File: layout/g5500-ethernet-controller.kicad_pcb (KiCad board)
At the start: 2 copper layers, 58 parts, among them IC1 MAX-M8Q, J1 CONN_01x03, J2 CONN_01x03, J3 MICROUSB, J4 CONN_01x02, J5 CONN_01x03, J6 CONN_01x03, K1 G5LE-1, K2 G5LE-1, K3 G5LE-1, K4 G5LE-1, P1 COAX, Q1 BC817W, Q2 BC817W, Q3 BC817W, Q4 BC817W, U1 NUCLEO144-F429ZI, U2 LD3985G33R_TSOT23

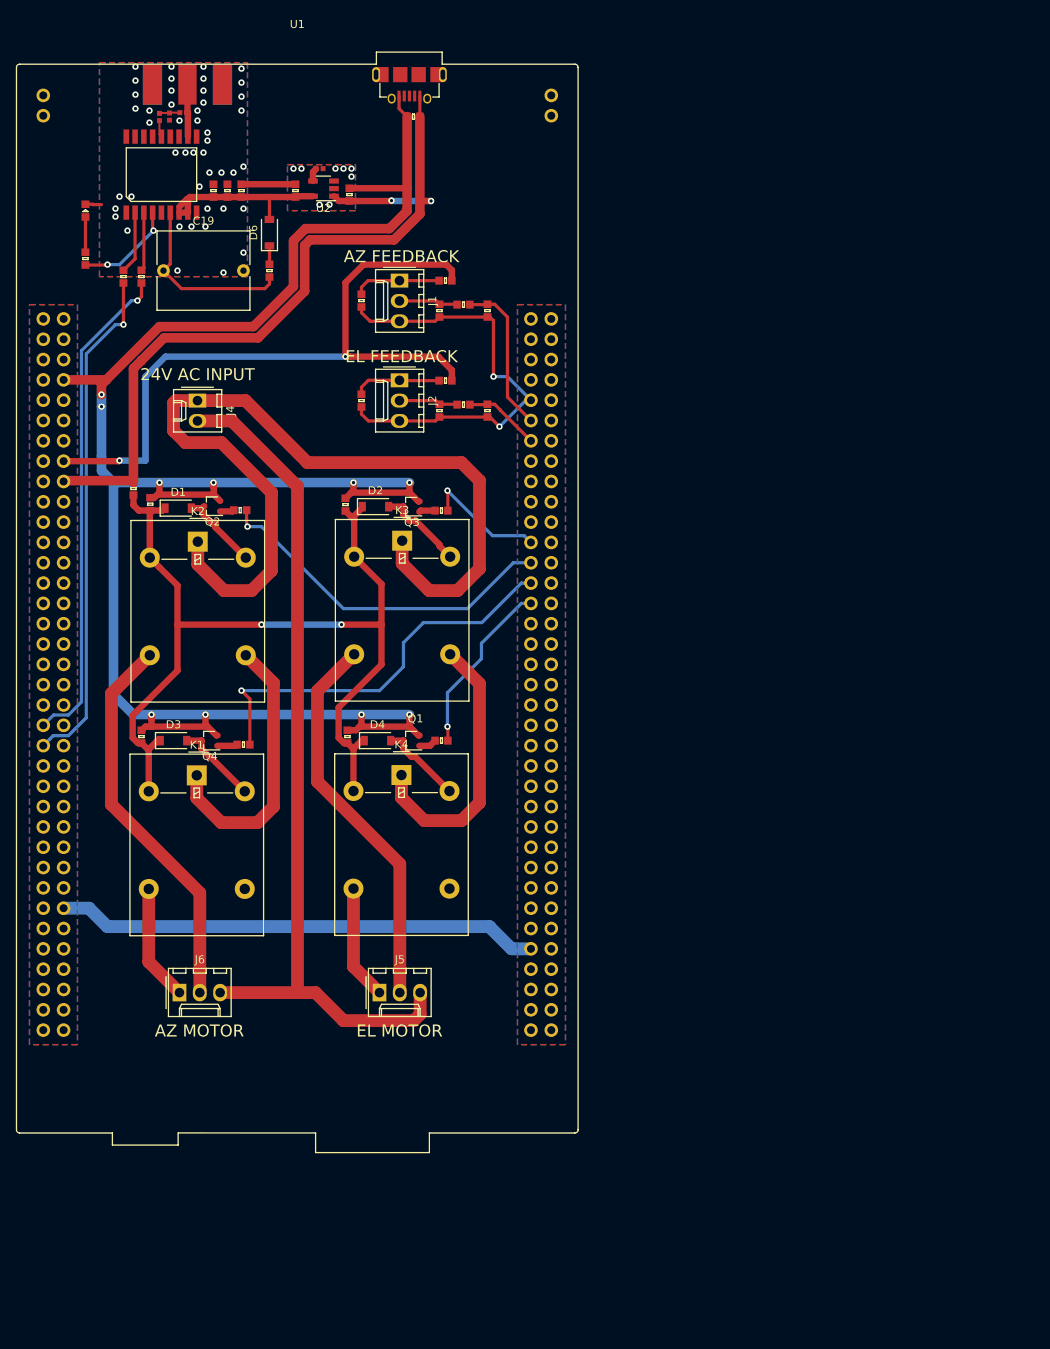
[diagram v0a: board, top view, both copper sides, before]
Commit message: Layout nearly done.
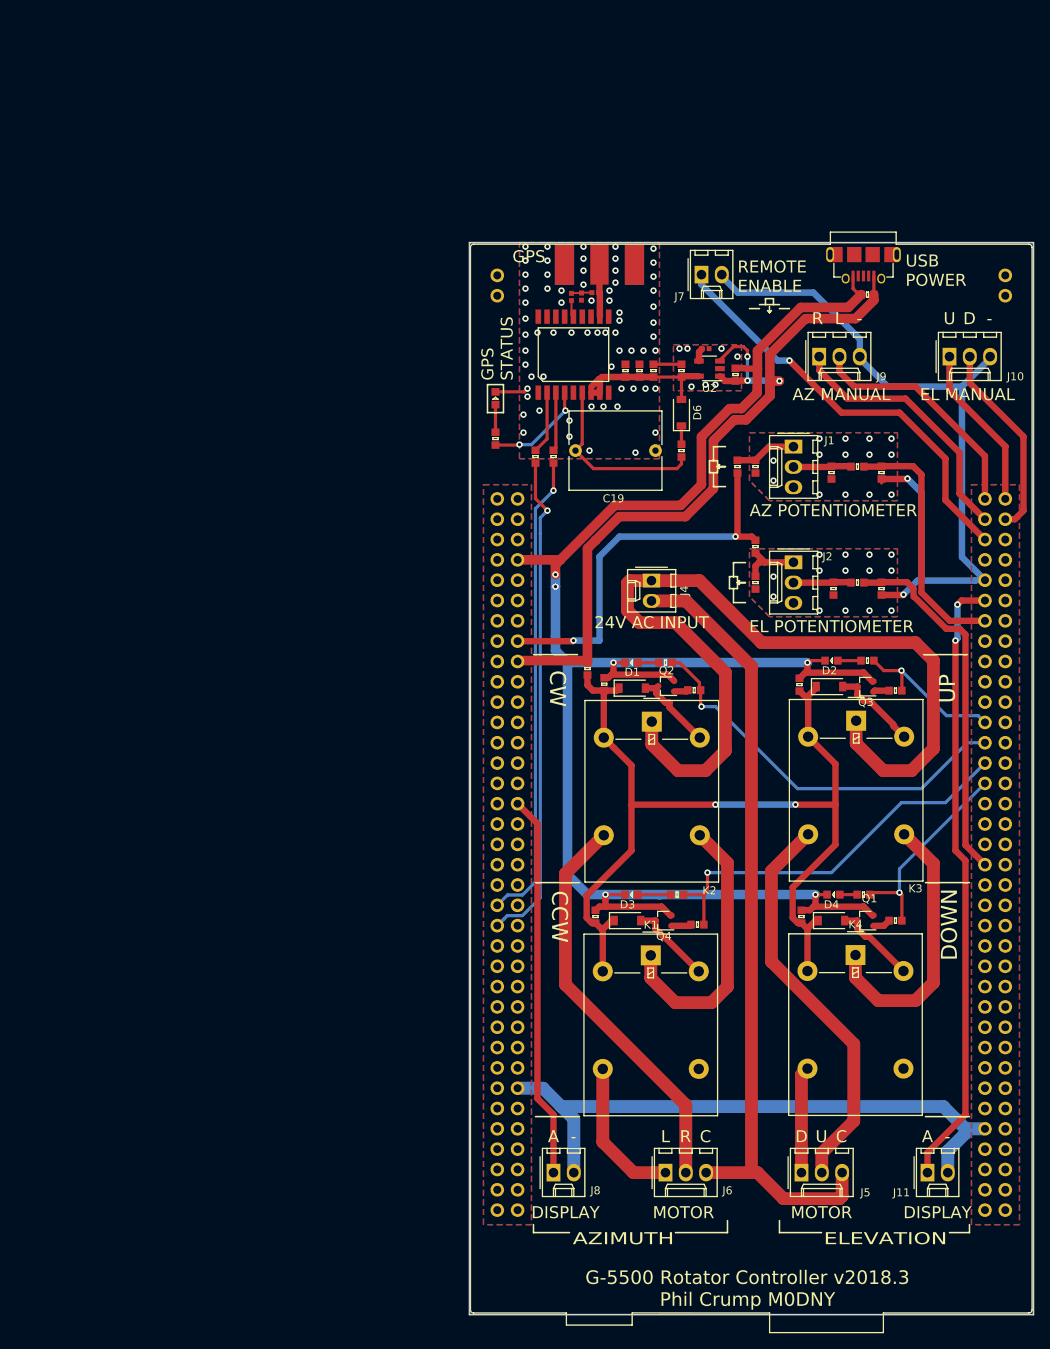
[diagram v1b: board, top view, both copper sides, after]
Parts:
- added D10: LED, agg:0603-LED, F.Cu at (77.5, 109.8)
- added D7: LED, agg:0603-LED, F.Cu at (102.8, 109.8)
- added D8: LED, agg:0603-LED, F.Cu at (77.5, 80.8)
- added D9: LED, agg:0603-LED, F.Cu at (102.5, 80.5)
- added J10: CONN_01x03, Connector_Molex:Molex_KK-254_AE-6410-03A_1x03_P2.54mm_Vertical, F.Cu at (117.2, 42.5)
- added J11: CONN_01x02, Connector_Molex:Molex_KK-254_AE-6410-02A_1x02_P2.54mm_Vertical, F.Cu at (114.5, 144.5)
- added J7: CONN_01x02, Connector_Molex:Molex_KK-254_AE-6410-02A_1x02_P2.54mm_Vertical, F.Cu at (86.2, 32.2)
- added J8: CONN_01x02, Connector_Molex:Molex_KK-254_AE-6410-02A_1x02_P2.54mm_Vertical, F.Cu at (67.8, 144.5)
- added J9: CONN_01x03, Connector_Molex:Molex_KK-254_AE-6410-03A_1x03_P2.54mm_Vertical, F.Cu at (101.0, 42.5)
- added R15: 1K, agg:0603, F.Cu at (106.5, 109.8)
- added R16: 1K, agg:0603, F.Cu at (81.8, 80.8)
- added R17: 1K, agg:0603, F.Cu at (107.0, 80.5)
- added R18: 1K, agg:0603, F.Cu at (83.2, 109.8)
- moved J6 64.8 mm to (81.8, 144.5)
- moved C9 61.0 mm to (74.1, 83.4)
- moved D1 61.0 mm to (77.6, 83.9)
- moved Q2 61.0 mm to (81.8, 83.7)
- moved R6 61.0 mm to (85.3, 84.2)
- moved C10 61.0 mm to (98.5, 83.5)
- moved C11 61.0 mm to (73.0, 112.5)
- moved C8 61.0 mm to (98.8, 112.5)
- moved D2 61.0 mm to (102.2, 83.8)
- moved D3 61.0 mm to (77.0, 113.0)
- moved D4 61.0 mm to (102.5, 113.0)
- moved J3 61.0 mm to (106.5, 29.8)
- moved J4 61.0 mm to (80.0, 70.5)
- moved K1 61.0 mm to (79.9, 117.3)
- moved K2 61.0 mm to (80.0, 88.1)
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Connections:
- D2 pad 2: /RELAY_DOWN -> /RELAY_UP
- D4 pad 2: /RELAY_UP -> /RELAY_DOWN
- K3 pad 5: /RELAY_DOWN -> /RELAY_UP
- K4 pad 5: /RELAY_UP -> /RELAY_DOWN
- Q1 pad 3: /RELAY_UP -> /RELAY_DOWN
- Q3 pad 3: /RELAY_DOWN -> /RELAY_UP
- R5 pad 1: /STM_EL_UP -> /STM_EL_DN
- R7 pad 1: /STM_EL_DN -> /STM_EL_UP
- U1 pad 101: /STM_EL_UP -> /STM_EL_DN
- U1 pad 109: Net-(U1-Pad109) -> /STM_EL_ANALOG
- U1 pad 32: Net-(U1-Pad32) -> /AZ_METER
- U1 pad 73: Net-(U1-Pad73) -> /AZ_CCW_SWITCH
- U1 pad 74: Net-(U1-Pad74) -> /EL_UP_SWITCH
- U1 pad 75: Net-(U1-Pad75) -> /AZ_CW_SWITCH
- U1 pad 76: Net-(U1-Pad76) -> /EL_DN_SWITCH
- U1 pad 77: Net-(U1-Pad77) -> /ENABLE_SWITCH
- U1 pad 83: /STM_AZ_ANALOG -> /EL_METER
- U1 pad 85: /STM_EL_ANALOG -> /STM_AZ_ANALOG
- U1 pad 95: /STM_EL_DN -> /STM_EL_UP
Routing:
- net /EL_METER: track 0.00 -> 77.2 mm, vias 0 -> 2
- net /ENABLE_SWITCH: track 0.00 -> 53.2 mm, vias 0 -> 1
- net /AZ_METER: track 0.00 -> 48.0 mm
- net GND: track 368.1 -> 406.6 mm, vias 66 -> 109
- net 3v3: track 87.2 -> 49.5 mm
- net /STM_EL_ANALOG: track 9.58 -> 45.7 mm
- net /AZ_CW_SWITCH: track 0.00 -> 33.2 mm
- net /AZ_CCW_SWITCH: track 0.00 -> 29.8 mm
- net /EL_DN_SWITCH: track 0.00 -> 24.8 mm
- net /EL_UP_SWITCH: track 0.00 -> 20.7 mm
- net /STM_AZ_ANALOG: track 19.6 -> 31.8 mm
- net /STM_EL_DN: track 15.6 -> 25.5 mm
- net Net-(J4-Pad2): track 108.6 -> 100.6 mm
- net /STM_AZ_CW: track 44.2 -> 49.6 mm
- net Net-(D10-Pad2): track 0.00 -> 4.10 mm
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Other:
- board outline added: 70.5 x 134 mm
- board text added: "-"
- board text added: "A"
- board text added: "AZ MANUAL"
- board text added: "AZ POTENTIOMETER"
- board text added: "AZIMUTH"
- board text added: "C"
- board text added: "CCW"
- board text added: "CW"
- board text added: "D"
- board text added: "DISPLAY"
- board text added: "DOWN"
- board text added: "EL MANUAL"
- board text added: "EL POTENTIOMETER"
- board text added: "ELEVATION"
- board text added: "G-5500 Rotator Controller v2018.3 Phil Crump M0DNY"
- board text added: "GPS"
- board text added: "GPS STATUS"
- board text added: "L"
- board text added: "MOTOR"
- board text added: "R"
- board text added: "REMOTE ENABLE"
- board text added: "U"
- board text added: "UP"
- board text added: "USB POWER"
- board text removed: "AZ FEEDBACK"
- board text removed: "AZ MOTOR"
- board text removed: "EL FEEDBACK"
- board text removed: "EL MOTOR"

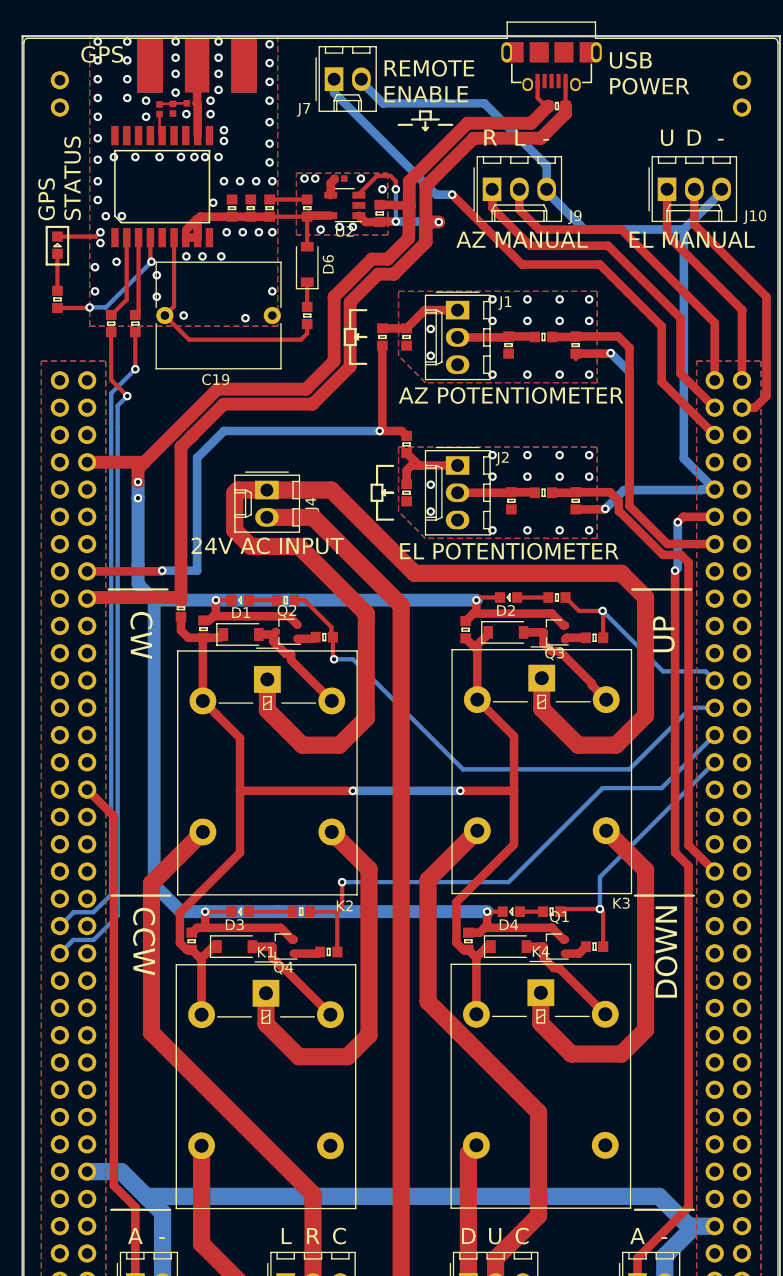
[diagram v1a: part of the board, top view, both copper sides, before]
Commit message: layout: Finish and send off v1.
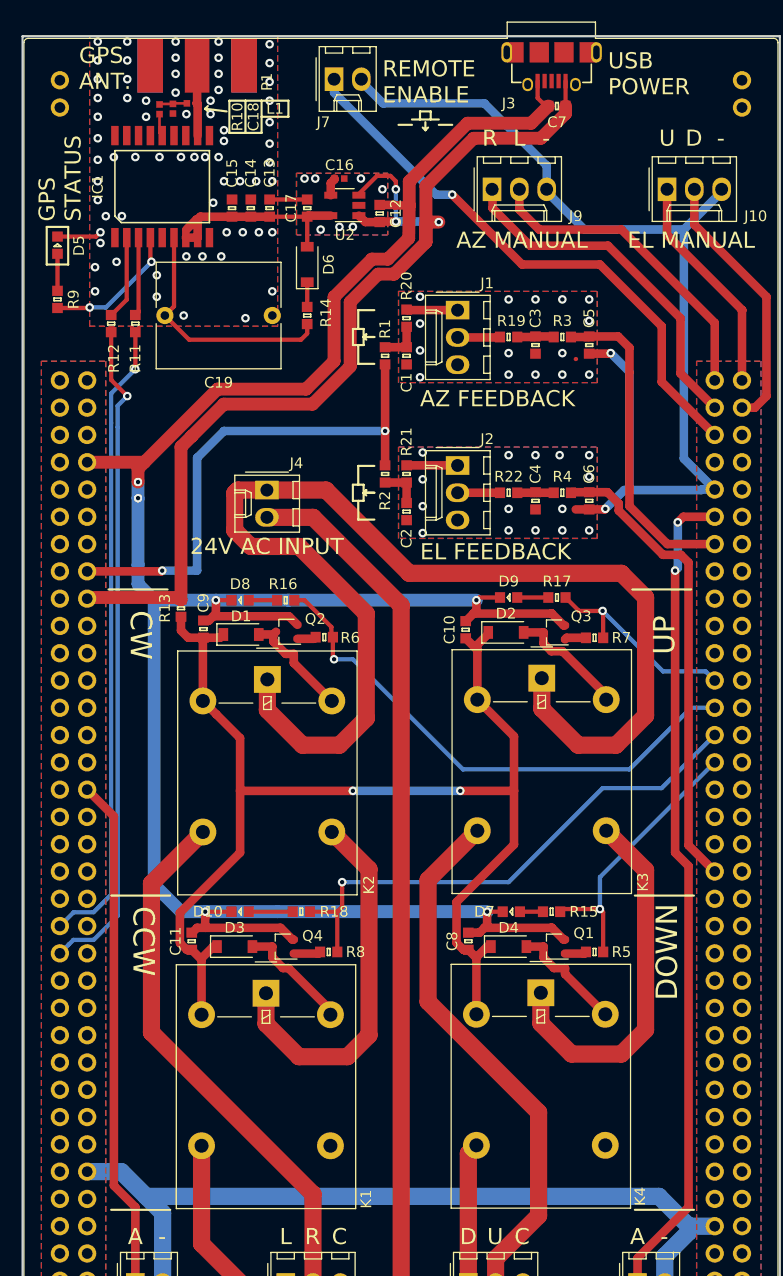
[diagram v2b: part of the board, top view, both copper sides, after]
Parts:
- added R19: 1K, agg:0603, F.Cu at (102.5, 56.2)
- added R20: 22R, agg:0603, F.Cu at (93.0, 54.5)
- added R21: 22R, agg:0603, F.Cu at (93.0, 69.0)
- added R22: 1K, agg:0603, F.Cu at (102.5, 70.8)
- R1, R2: value 100R -> 22R
- moved R2 3.40 mm to (91.0, 69.0)
- moved C3 2.50 mm to (105.0, 57.0)
- moved C4 2.25 mm to (105.0, 71.5)
- moved R1 1.77 mm to (91.0, 58.0)
- moved C1 1.75 mm to (93.0, 58.0)
- moved C2 1.75 mm to (93.0, 72.5)
- moved R3 1.75 mm to (107.5, 56.2)
- moved R4 1.75 mm to (107.5, 70.8)
- moved C5 1.25 mm to (110.0, 57.0)
- moved C6 1.25 mm to (110.0, 71.5)
- moved R5 0.50 mm to (110.5, 113.5)
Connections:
- J1 pad 1: Net-(C1-Pad1) -> Net-(J1-Pad1)
- J1 pad 2: Net-(C3-Pad1) -> Net-(J1-Pad2)
- J2 pad 1: Net-(C2-Pad1) -> Net-(J2-Pad1)
- J2 pad 2: Net-(C4-Pad1) -> Net-(J2-Pad2)
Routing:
- net Net-(J2-Pad1): track 0.00 -> 4.81 mm
- net Net-(J1-Pad1): track 0.00 -> 4.77 mm
- net Net-(C2-Pad1): track 7.91 -> 3.90 mm
- net Net-(J2-Pad2): track 0.00 -> 3.95 mm
- net Net-(C3-Pad1): track 7.26 -> 3.44 mm
- net Net-(C1-Pad1): track 7.70 -> 3.90 mm
- net Net-(C4-Pad1): track 7.24 -> 3.51 mm
- net Net-(J1-Pad2): track 0.00 -> 3.68 mm
- net /STM_EL_ANALOG: track 45.7 -> 43.8 mm
- net /STM_AZ_ANALOG: track 31.8 -> 30.1 mm
- net GND: track 406.6 -> 405.3 mm, vias 109 -> 111
- net 3v3: track 49.5 -> 48.7 mm
- net /STM_EL_DN: track 25.5 -> 26.0 mm
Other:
- board text added: "AZ FEEDBACK"
- board text added: "EL FEEDBACK"
- board text added: "GPS ANT."
- board text removed: "AZ POTENTIOMETER"
- board text removed: "EL POTENTIOMETER"
- board text removed: "GPS"
